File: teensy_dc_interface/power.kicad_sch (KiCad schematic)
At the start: 51 parts, among them U3 AP65211A, U4 AP62200TWU-7, U9 AP65211A

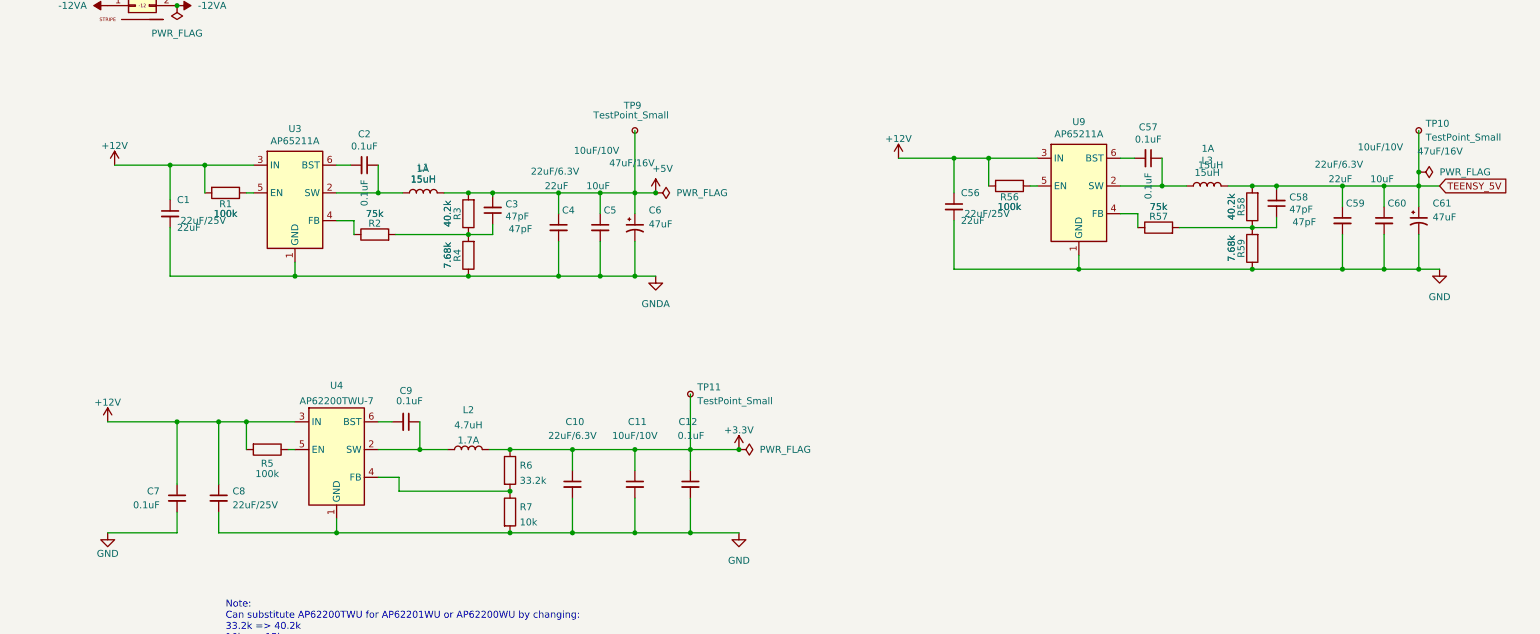
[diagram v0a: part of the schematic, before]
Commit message: Generated gerbers for boards
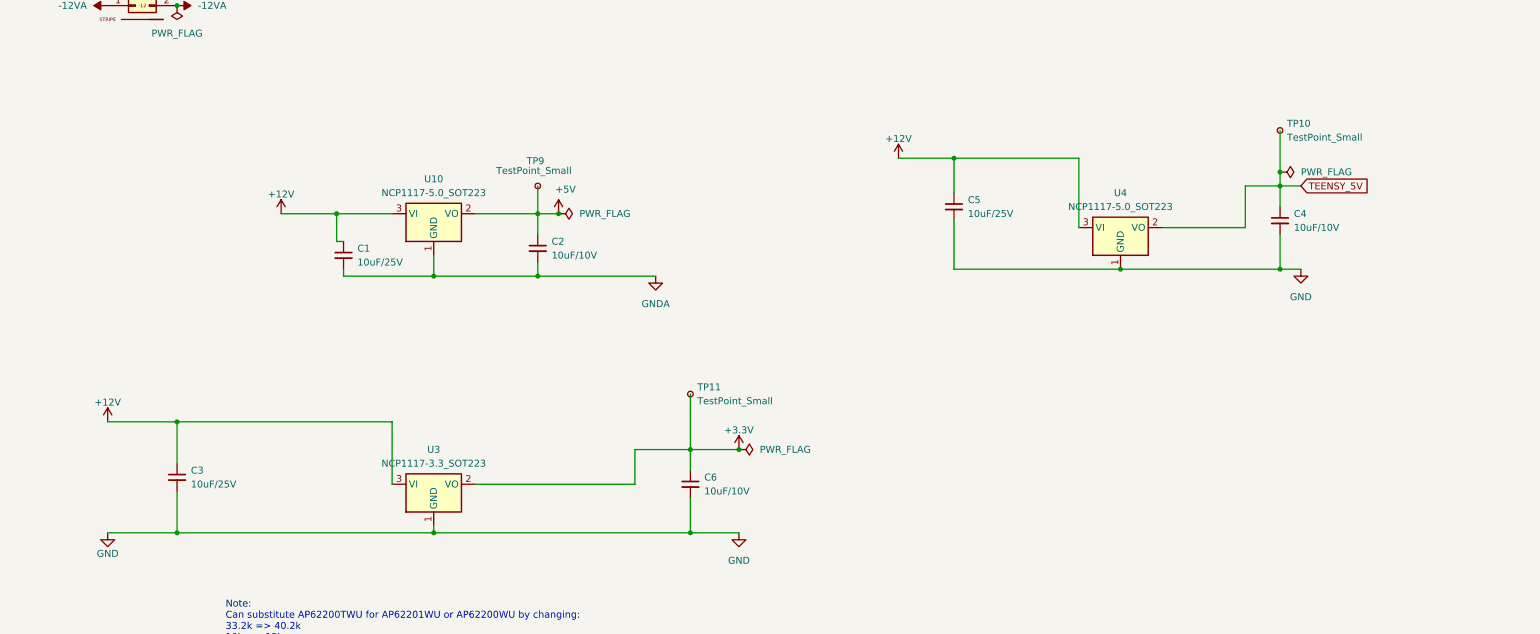
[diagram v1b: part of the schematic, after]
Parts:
- removed C1, C56: 22uF, 4ms_Capacitor:C_0805, symbol 4ms_Capacitor:22uF_0805_25V
- removed C10: 22uF_0805_6.3V, 4ms_Capacitor:C_0805, symbol 4ms_Capacitor:22uF_0805_6.3V
- removed C11: 10uF_0603_10V, 4ms_Capacitor:C_0603, symbol 4ms_Capacitor:10uF_0603_10V
- removed C12, C7, C9: 0.1uF_0603_16V, 4ms_Capacitor:C_0603, symbol 4ms_Capacitor:0.1uF_0603_16V
- removed C2, C57: 0.1uF, 4ms_Capacitor:C_0603, symbol 4ms_Capacitor:0.1uF_0603_16V
- removed C3, C58: 47pF, 4ms_Capacitor:C_0603, symbol 4ms_Capacitor:47pF_0603_50V
- removed C4, C59: 22uF, 4ms_Capacitor:C_0603, symbol 4ms_Capacitor:22uF_0603_6.3V
- removed C5, C60: 10uF, 4ms_Capacitor:C_0603, symbol 4ms_Capacitor:10uF_0603_10V
- removed C6, C61: 47uF, 4ms_Capacitor:CP_Elec_5x5.3, symbol 4ms_Capacitor:47uF_5x5.3_16V
- removed C8: 22uF_0805_25V, 4ms_Capacitor:C_0805, symbol 4ms_Capacitor:22uF_0805_25V
- removed L1, L3: 15uH, 4ms_Inductor:COIL_5040, symbol 4ms_Inductor:15uH_1A_5040
- removed L2: 4.7uH_1.2A_40xx, Inductor_SMD:L_Taiyo-Yuden_NR-40xx, symbol 4ms_Inductor:4.7uH_1.2A_40xx
- removed R1, R56: 100k, 4ms_Resistor:R_0603, symbol 4ms_Resistor_0603:100k_0603
- removed R2, R57: 75k, 4ms_Resistor:R_0603, symbol 4ms_Resistor:75k_0603
- removed R3, R58: 40.2k, 4ms_Resistor:R_0603, symbol 4ms_Resistor:40.2k_0603
- removed R4, R59: 7.68k, 4ms_Resistor:R_0603, symbol 4ms_Resistor:7.68k_0603
- removed R5: 100k_0603, 4ms_Resistor:R_0603, symbol 4ms_Resistor:100k_0603
- removed R6: 33.2k_0603, 4ms_Resistor:R_0603, symbol 4ms_Resistor:33.2k_0603
- removed R7: 10k_0603, 4ms_Resistor:R_0603, symbol 4ms_Resistor:10k_0603
- removed U3, U9: AP65211A, 4ms_Package_SOT:TSOT-23-6, symbol 4ms_IC:AP65211AWU-7
- removed U4: AP62200TWU-7, 4ms_Package_SOT:TSOT-23-6, symbol 4ms_IC:AP62200TWU-7
- added C1, C3, C5: 10uF_0805_25V, 4ms_Capacitor:C_0805, symbol 4ms_Capacitor:10uF_0805_25V
- added C2, C4, C6: 10uF_0603_10V, 4ms_Capacitor:C_0603, symbol 4ms_Capacitor:10uF_0603_10V
- added U10, U4: NCP1117-5.0_SOT223, Package_TO_SOT_SMD:SOT-223-3_TabPin2, symbol Regulator_Linear:NCP1117-5.0_SOT223
- added U3: NCP1117-3.3_SOT223, Package_TO_SOT_SMD:SOT-223-3_TabPin2, symbol Regulator_Linear:NCP1117-3.3_SOT223
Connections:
- net +12V: now also C1.1, C3.1, C5.1, U10.3 (VI), U3.3 (VI), U4.3 (VI)
- net +3.3V: now also C6.1, U3.2 (VO)
- net +5V: now also C2.1, U10.2 (VO)
- net GND: now also C3.2, C4.2, C5.2, C6.2, U3.1 (GND), U4.1 (GND)
- net GNDA: now also C1.2, C2.2, U10.1 (GND)
- net TEENSY_5V: now also C4.1, U4.2 (VO)
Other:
- moved on the sheet: TP10, TP9
